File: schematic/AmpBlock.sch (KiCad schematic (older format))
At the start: 14 parts, among them IC8 LTC6090CS8E#PBF

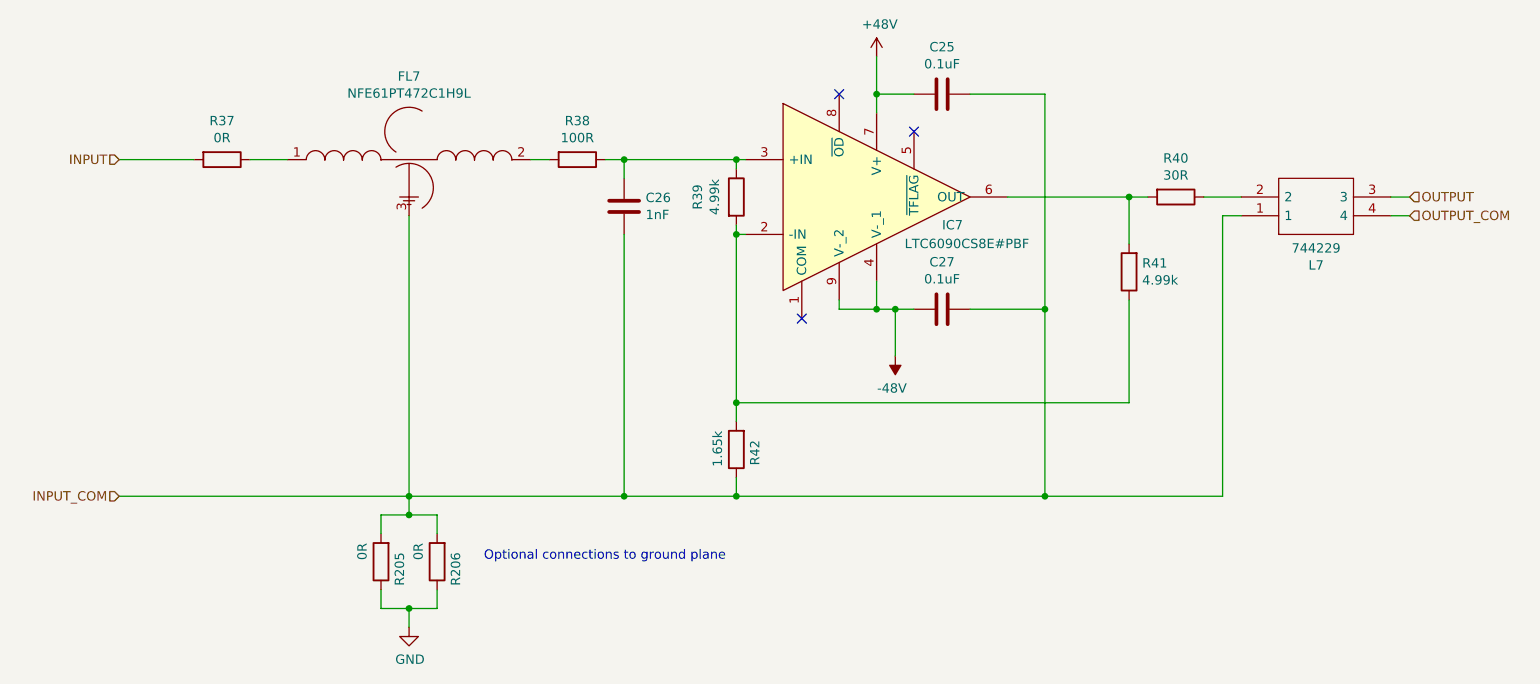
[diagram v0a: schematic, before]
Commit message: Penultimate tweaks
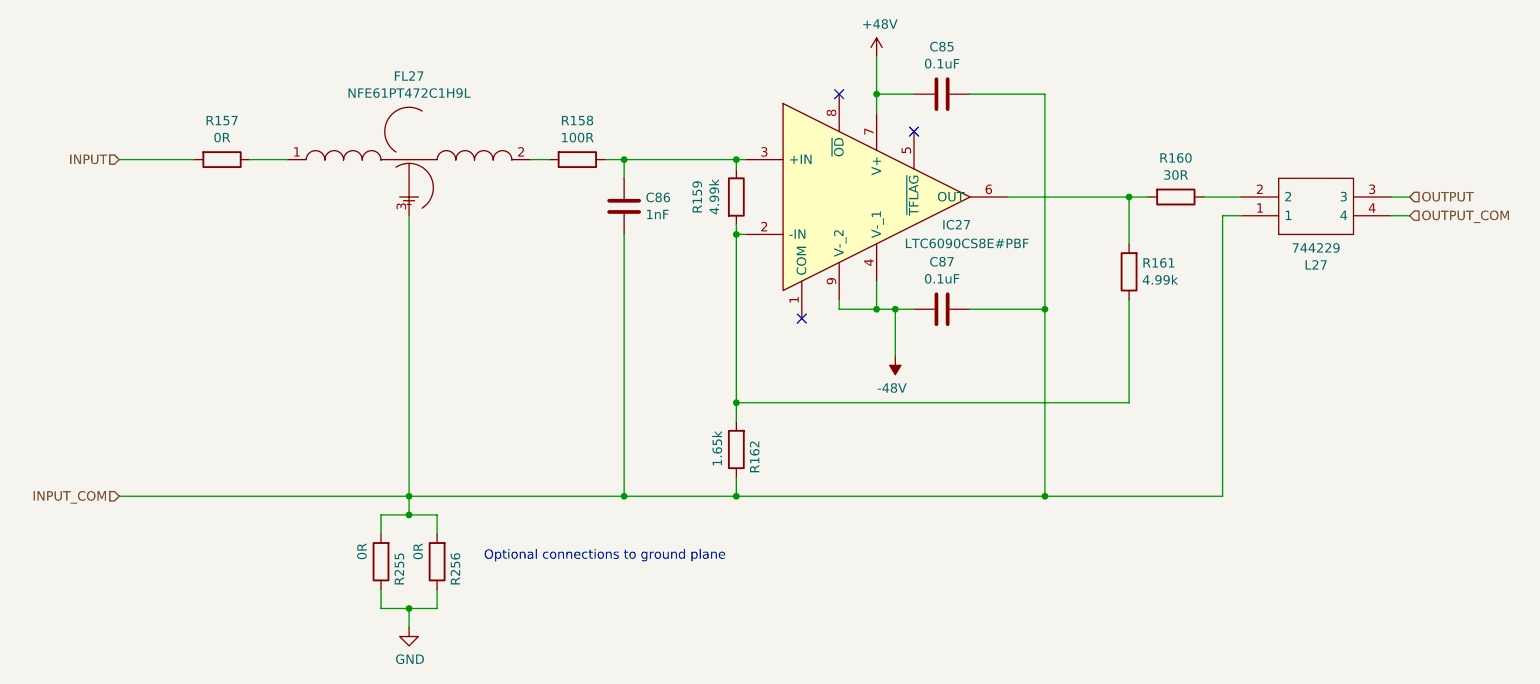
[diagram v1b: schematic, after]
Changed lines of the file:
@@
 AR Path="/5CAE2EB0/5FE9E532" Ref="R188"  Part="1"
 AR Path="/5FE9E532" Ref="R?"  Part="1"
-F 0 "R38" V 3743 3400 50  0000 C CNN
+F 0 "R158" V 3743 3400 50  0000 C CNN
 F 1 "100R" V 3834 3400 50  0000 C CNN
 F 2 "Resistor_SMD:R_0603_1608Metric" V 3880 3400 50  0001 C CNN
@@
 AR Path="/5CAE2EB0/5C969C02" Ref="R192"  Part="1"
 AR Path="/5C969C02" Ref="R?"  Part="1"
-F 0 "R42" V 4700 4900 50  0000 L CNN
+F 0 "R162" V 4700 4900 50  0000 L CNN
 F 1 "1.65k" V 4900 4850 50  0000 L CNN
 F 2 "Resistor_SMD:R_0603_1608Metric" V 4730 4950 50  0001 C CNN
@@
 AR Path="/5CAE2EB0/5C96A29C" Ref="R191"  Part="1"
 AR Path="/5C96A29C" Ref="R?"  Part="1"
-F 0 "R41" H 6830 3954 50  0000 R CNN
+F 0 "R161" H 6830 3954 50  0000 R CNN
 F 1 "4.99k" H 6830 4045 50  0000 R CNN
 F 2 "Resistor_SMD:R_0603_1608Metric" V 6830 4000 50  0001 C CNN
@@
 AR Path="/5CAE2EB0/5C96A628" Ref="C101"  Part="1"
 AR Path="/5C96A628" Ref="C?"  Part="1"
-F 0 "C26" H 4315 3696 50  0000 L CNN
+F 0 "C86" H 4315 3696 50  0000 L CNN
 F 1 "1nF" H 4315 3605 50  0000 L CNN
 F 2 "Capacitor_SMD:C_0603_1608Metric" H 4238 3500 50  0001 C CNN
@@
 AR Path="/5CAE2EB0/5C96EFD0" Ref="#PWR073"  Part="1"
 AR Path="/5C96EFD0" Ref="#PWR?"  Part="1"
-F 0 "#PWR023" H 5550 2700 50  0001 C CNN
+F 0 "#PWR063" H 5550 2700 50  0001 C CNN
 F 1 "+48V" H 5567 3023 50  0000 C CNN
 F 2 "" H 5550 2850 50  0001 C CNN
@@
 AR Path="/5CAE2EB0/5FE9E537" Ref="#PWR074"  Part="1"
 AR Path="/5FE9E537" Ref="#PWR?"  Part="1"
-F 0 "#PWR024" H 5650 4300 50  0001 C CNN
+F 0 "#PWR064" H 5650 4300 50  0001 C CNN
 F 1 "-48V" H 5668 4623 50  0000 C CNN
 F 2 "" H 5650 4450 50  0001 C CNN
@@
 AR Path="/5CAE2EB0/5C96FD85" Ref="C100"  Part="1"
 AR Path="/5C96FD85" Ref="C?"  Part="1"
-F 0 "C25" V 5648 3050 50  0000 C CNN
+F 0 "C85" V 5648 3050 50  0000 C CNN
 F 1 "0.1uF" V 5739 3050 50  0000 C CNN
 F 2 "Capacitor_SMD:C_0603_1608Metric" H 5938 2900 50  0001 C CNN
@@
 AR Path="/5CAE2EB0/5FE9E539" Ref="C102"  Part="1"
 AR Path="/5FE9E539" Ref="C?"  Part="1"
-F 0 "C27" V 5648 4200 50  0000 C CNN
+F 0 "C87" V 5648 4200 50  0000 C CNN
 F 1 "0.1uF" V 5739 4200 50  0000 C CNN
 F 2 "Capacitor_SMD:C_0603_1608Metric" H 5938 4050 50  0001 C CNN
@@
 AR Path="/5CAE2E6A/5E7F6ABF" Ref="FL31"  Part="1"
 AR Path="/5CAE2EB0/5E7F6ABF" Ref="FL32"  Part="1"
-F 0 "FL7" H 3050 3845 50  0000 C CNN
+F 0 "FL27" H 3050 3845 50  0000 C CNN
 F 1 "NFE61PT472C1H9L" H 3050 3754 50  0000 C CNN
 F 2 "ARTIQAmp:NFE61" H 3400 3650 50  0001 L CNN
@@
 AR Path="/5CAE2EB0/5F650121" Ref="R187"  Part="1"
 AR Path="/5F650121" Ref="R?"  Part="1"
-F 0 "R37" V 1843 3400 50  0000 C CNN
+F 0 "R157" V 1843 3400 50  0000 C CNN
 F 1 "0R" V 1934 3400 50  0000 C CNN
 F 2 "Resistor_SMD:R_0603_1608Metric" V 1980 3400 50  0001 C CNN
@@
 AR Path="/5CAE2EB0/5F6588CE" Ref="R189"  Part="1"
 AR Path="/5F6588CE" Ref="R?"  Part="1"
-F 0 "R39" V 4593 3600 50  0000 C CNN
+F 0 "R159" V 4593 3600 50  0000 C CNN
 F 1 "4.99k" V 4684 3600 50  0000 C CNN
 F 2 "Resistor_SMD:R_0603_1608Metric" V 4730 3600 50  0001 C CNN
@@
 AR Path="/5CAE2EB0/5F678EAA" Ref="R190"  Part="1"
 AR Path="/5F678EAA" Ref="R?"  Part="1"
-F 0 "R40" V 6943 3600 50  0000 C CNN
+F 0 "R160" V 6943 3600 50  0000 C CNN
 F 1 "30R" V 7034 3600 50  0000 C CNN
 F 2 "Resistor_SMD:R_0603_1608Metric" V 7080 3600 50  0001 C CNN
@@
 AR Path="/5CAE2E6A/5F68D18B" Ref="L31"  Part="1"
 AR Path="/5CAE2EB0/5F68D18B" Ref="L32"  Part="1"
-F 0 "L7" H 7900 3965 50  0000 C CNN
+F 0 "L27" H 7900 3965 50  0000 C CNN
 F 1 "744229" H 7900 3874 50  0000 C CNN
 F 2 "ARTIQAmp:WE-SL2" H 8150 3800 50  0001 L CNN
@@
 AR Path="/5CAE2E6A/5F68D7CC" Ref="IC31"  Part="1"
 AR Path="/5CAE2EB0/5F68D7CC" Ref="IC32"  Part="1"
-F 0 "IC7" H 5900 3450 50  0000 L CNN
+F 0 "IC27" H 5900 3450 50  0000 L CNN
 F 1 "LTC6090CS8E#PBF" H 5700 3350 50  0000 L CNN
 F 2 "ARTIQAmp:SOIC127P599X175-9N" H 5600 4200 50  0001 L CNN
@@
 AR Path="/5CAE2EB0/5F8DFD1E" Ref="#PWR0135"  Part="1"
 AR Path="/5CAE2E52/5F8DFD1E" Ref="#PWR0136"  Part="1"
-F 0 "#PWR0111" H 3050 5650 50  0001 C CNN
+F 0 "#PWR0136" H 3050 5650 50  0001 C CNN
 F 1 "GND" H 3055 5727 50  0000 C CNN
 F 2 "" H 3050 5900 50  0001 C CNN
@@
 AR Path="/5CAE2EB0/5F8E08A0" Ref="R253"  Part="1"
 AR Path="/5F8E08A0" Ref="R?"  Part="1"
-F 0 "R205" V 2800 5500 50  0000 L CNN
+F 0 "R255" V 2800 5500 50  0000 L CNN
 F 1 "0R" V 3000 5450 50  0000 L CNN
 F 2 "Resistor_SMD:R_0603_1608Metric" V 2830 5550 50  0001 C CNN
@@
 AR Path="/5CAE2EB0/5F8E1BE6" Ref="R254"  Part="1"
 AR Path="/5F8E1BE6" Ref="R?"  Part="1"
-F 0 "R206" V 3100 5500 50  0000 L CNN
+F 0 "R256" V 3100 5500 50  0000 L CNN
 F 1 "0R" V 3300 5450 50  0000 L CNN
 F 2 "Resistor_SMD:R_0603_1608Metric" V 3130 5550 50  0001 C CNN
